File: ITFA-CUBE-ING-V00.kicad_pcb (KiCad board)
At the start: 2 copper layers, 90.2 x 95.9 mm, 34 parts, among them J1 Conn_01x04, U1 STM32H743VITx, U2 W25Q128JVS, Y1 25MHz 10pF, Y2 32.768K 7pF

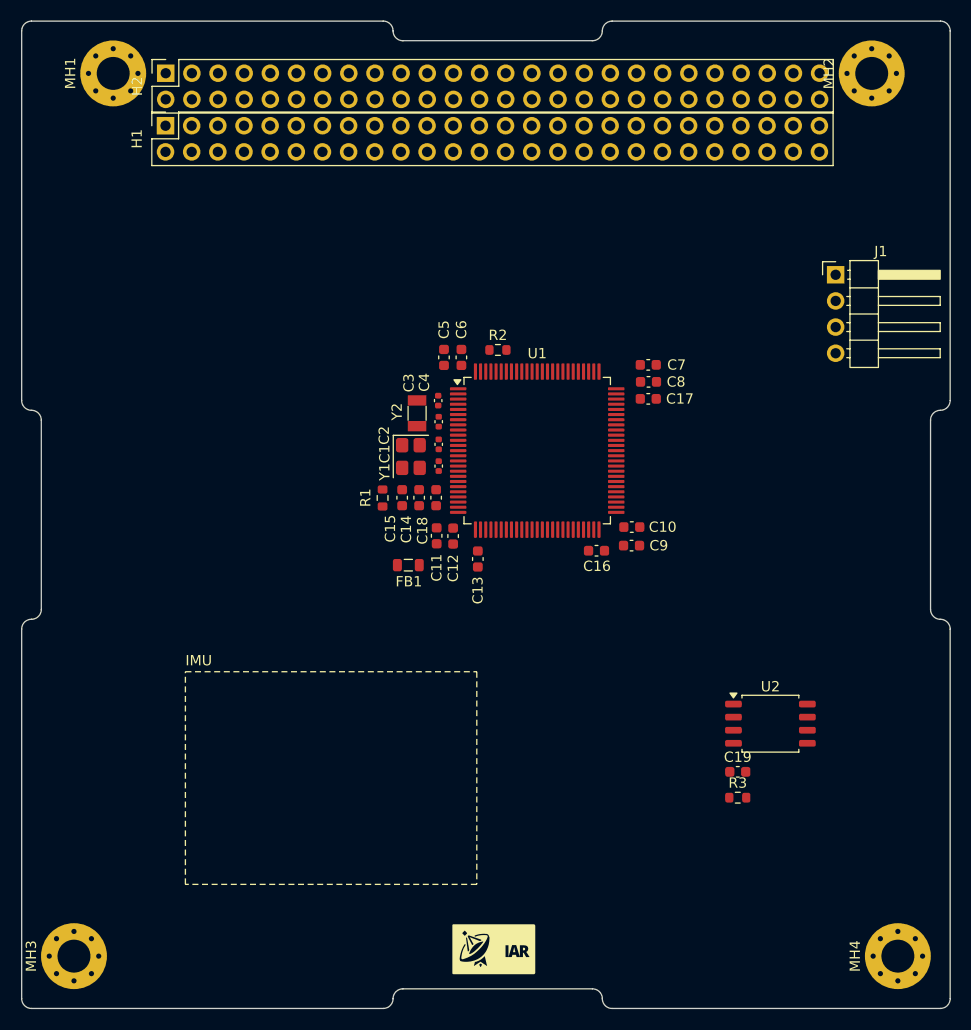
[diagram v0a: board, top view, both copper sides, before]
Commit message: Avance uc
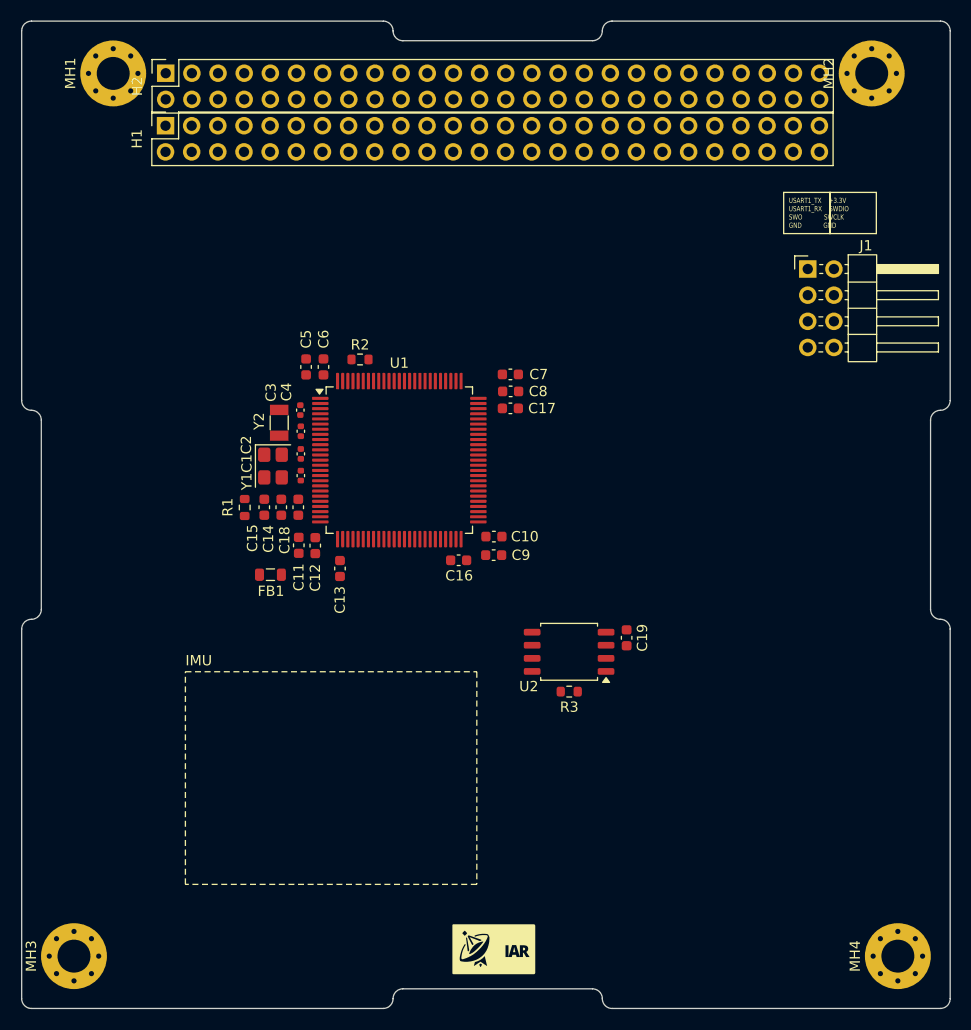
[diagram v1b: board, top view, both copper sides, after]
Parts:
- J1: value Conn_01x04 -> Conn_02x04_Odd_Even; footprint Connector_PinHeader_2.54mm:PinHeader_1x04_P2.54mm_Horizontal -> Connector_PinHeader_2.54mm:PinHeader_2x04_P2.54mm_Horizontal
- moved U2 20.8 mm to (139.8, 106.1), turned to 180 degrees
- moved R3 19.3 mm to (139.8, 110.0), turned to 180 degrees
- moved C19 16.9 mm to (145.4, 104.7), turned to 90 degrees
- moved C10 13.4 mm to (132.5, 94.9)
- moved C7 13.4 mm to (134.1, 79.2)
- moved C16 13.4 mm to (129.0, 97.2)
- moved C17 13.4 mm to (134.1, 82.5)
- moved C8 13.4 mm to (134.1, 80.8)
- moved C9 13.4 mm to (132.4, 96.7)
- moved R2 13.4 mm to (119.5, 77.7)
- moved U1 13.4 mm to (123.3, 87.5)
- moved C1 13.4 mm to (113.7, 86.9)
- moved C4 13.4 mm to (113.7, 82.6)
- moved C11 13.4 mm to (113.5, 95.8)
- moved C13 13.4 mm to (117.5, 98.0)
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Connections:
- net Net-(U1-PC14) renamed /RCC_OSC32_IN
- net Net-(U1-PC15) renamed /RCC_OSC32_OUT
- H1 pad 10: SPI_1_MOSI -> unconnected-(H1-Pin_10-Pad10)
- H1 pad 11: SPI_1_SCK -> unconnected-(H1-Pin_11-Pad11)
- H1 pad 12: SPI_1_MISO -> unconnected-(H1-Pin_12-Pad12)
- H1 pad 13: UART_1_TX -> unconnected-(H1-Pin_13-Pad13)
- H1 pad 14: UART_1_CTS -> unconnected-(H1-Pin_14-Pad14)
- H1 pad 15: UART_1_RX -> unconnected-(H1-Pin_15-Pad15)
- H1 pad 16: UART_1_RST -> unconnected-(H1-Pin_16-Pad16)
- H1 pad 17: UART_RCS_1_TX -> unconnected-(H1-Pin_17-Pad17)
- H1 pad 18: UART_RCS_1_CTS -> unconnected-(H1-Pin_18-Pad18)
- H1 pad 19: UART_RCS_1_RX -> unconnected-(H1-Pin_19-Pad19)
- H1 pad 20: UART_RCS_1_RST -> unconnected-(H1-Pin_20-Pad20)
- H1 pad 21: I2C_1_SCL -> unconnected-(H1-Pin_21-Pad21)
- H1 pad 22: I2C_1_SDA -> unconnected-(H1-Pin_22-Pad22)
- H1 pad 23: CAN_1_P -> unconnected-(H1-Pin_23-Pad23)
- H1 pad 24: CAN_1_N -> unconnected-(H1-Pin_24-Pad24)
- H1 pad 25: GLO_SYNC -> unconnected-(H1-Pin_25-Pad25)
- H1 pad 26: GLO_FAULT -> unconnected-(H1-Pin_26-Pad26)
- H1 pad 27: CPU_WD_1 -> unconnected-(H1-Pin_27-Pad27)
- H1 pad 30: CPU_MODE -> unconnected-(H1-Pin_30-Pad30)
- H1 pad 35: GLO_KS_1 -> unconnected-(H1-Pin_35-Pad35)
- H1 pad 39: USER_3_1 -> unconnected-(H1-Pin_39-Pad39)
- H1 pad 40: USER_3_2 -> unconnected-(H1-Pin_40-Pad40)
- H1 pad 41: USER_3_3 -> unconnected-(H1-Pin_41-Pad41)
- H1 pad 42: USER_3_4 -> unconnected-(H1-Pin_42-Pad42)
- H1 pad 43: USER_5_1 -> unconnected-(H1-Pin_43-Pad43)
- H1 pad 44: USER_5_2 -> unconnected-(H1-Pin_44-Pad44)
- H1 pad 45: USER_5_3 -> unconnected-(H1-Pin_45-Pad45)
- H1 pad 46: USER_5_4 -> unconnected-(H1-Pin_46-Pad46)
- H1 pad 5: USER_1_1 -> unconnected-(H1-Pin_5-Pad5)
- H1 pad 6: USER_1_2 -> unconnected-(H1-Pin_6-Pad6)
- H1 pad 7: SPI_1_CS2 -> unconnected-(H1-Pin_7-Pad7)
- H1 pad 8: USER_1_4 -> unconnected-(H1-Pin_8-Pad8)
- H1 pad 9: SPI_1_CS1 -> unconnected-(H1-Pin_9-Pad9)
- H2 pad 10: SPI_2_MOSI -> unconnected-(H2-Pin_10-Pad10)
- H2 pad 11: SPI_2_SCK -> unconnected-(H2-Pin_11-Pad11)
- H2 pad 12: SPI_2_MISO -> unconnected-(H2-Pin_12-Pad12)
- H2 pad 13: UART_2_TX -> unconnected-(H2-Pin_13-Pad13)
- H2 pad 14: UART_2_CTS -> unconnected-(H2-Pin_14-Pad14)
- H2 pad 15: UART_2_RX -> unconnected-(H2-Pin_15-Pad15)
- H2 pad 16: UART_2_RST -> unconnected-(H2-Pin_16-Pad16)
- H2 pad 17: UART_RCS_2_TX -> unconnected-(H2-Pin_17-Pad17)
- H2 pad 18: UART_RCS_2_CTS -> unconnected-(H2-Pin_18-Pad18)
- H2 pad 19: UART_RCS_2_RX -> unconnected-(H2-Pin_19-Pad19)
- H2 pad 20: UART_RCS_2_RST -> unconnected-(H2-Pin_20-Pad20)
- H2 pad 21: I2C_2_SCL -> unconnected-(H2-Pin_21-Pad21)
- H2 pad 22: I2C_2_SDA -> unconnected-(H2-Pin_22-Pad22)
- H2 pad 23: CAN_2_P -> unconnected-(H2-Pin_23-Pad23)
- H2 pad 24: CAN_2_N -> unconnected-(H2-Pin_24-Pad24)
- H2 pad 25: SUP_5V -> unconnected-(H2-Pin_25-Pad25)
- H2 pad 26: SUP_5V -> unconnected-(H2-Pin_26-Pad26)
- H2 pad 27: SUP_3V3 -> unconnected-(H2-Pin_27-Pad27)
- H2 pad 28: SUP_3V3 -> unconnected-(H2-Pin_28-Pad28)
- H2 pad 39: USER_4_1 -> unconnected-(H2-Pin_39-Pad39)
- H2 pad 40: USER_4_2 -> unconnected-(H2-Pin_40-Pad40)
- H2 pad 41: USER_4_3 -> unconnected-(H2-Pin_41-Pad41)
- H2 pad 42: USER_4_4 -> unconnected-(H2-Pin_42-Pad42)
- H2 pad 43: USER_6_1 -> unconnected-(H2-Pin_43-Pad43)
- H2 pad 44: USER_6_2 -> unconnected-(H2-Pin_44-Pad44)
- H2 pad 47: USER_6_3 -> unconnected-(H2-Pin_47-Pad47)
- H2 pad 48: USER_6_4 -> unconnected-(H2-Pin_48-Pad48)
- H2 pad 5: USER_2_1 -> unconnected-(H2-Pin_5-Pad5)
- H2 pad 6: USER_2_2 -> unconnected-(H2-Pin_6-Pad6)
- H2 pad 7: SPI_2_CS2 -> unconnected-(H2-Pin_7-Pad7)
- H2 pad 8: USER_2_4 -> unconnected-(H2-Pin_8-Pad8)
- H2 pad 9: SPI_2_CS1 -> unconnected-(H2-Pin_9-Pad9)
- J1 pad 1: +3.3V -> /USART1_TX
- J1 pad 2: /SWDIO -> +3.3V
- J1 pad 3: /SWCLK -> /USART1_RX
- J1 pad 4: GND -> /SWDIO
- R3 pad 1: /SPI_Flash_CS -> /SPI1_Flash1_CS
- U1 pad 1: unconnected-(U1-PE2-Pad1) -> /SPI4_CLK
- U1 pad 24: unconnected-(U1-PA2-Pad24) -> /USART2_TX
- U1 pad 25: unconnected-(U1-PA3-Pad25) -> /USART2_RX
- U1 pad 28: unconnected-(U1-PA4-Pad28) -> /SPI1_Flash1_CS
- U1 pad 29: unconnected-(U1-PA5-Pad29) -> /SPI1_CLK
- U1 pad 30: unconnected-(U1-PA6-Pad30) -> /SPI1_MISO
- U1 pad 31: unconnected-(U1-PA7-Pad31) -> /SPI1_MOSI
- U1 pad 4: unconnected-(U1-PE5-Pad4) -> /SPI4_MISO
- U1 pad 46: unconnected-(U1-PB10-Pad46) -> /I2C2_SCL
- U1 pad 47: unconnected-(U1-PB11-Pad47) -> /I2C2_SDA
- U1 pad 5: unconnected-(U1-PE6-Pad5) -> /SPI4_MOSI
- U1 pad 68: unconnected-(U1-PA9-Pad68) -> /USART1_TX
- U1 pad 69: unconnected-(U1-PA10-Pad69) -> /USART1_RX
- U1 pad 89: unconnected-(U1-PB3-Pad89) -> /SWO
- U1 pad 92: unconnected-(U1-PB6-Pad92) -> /I2C1_SCL
- U1 pad 93: unconnected-(U1-PB7-Pad93) -> /I2C1_SDA
- U1 pad 95: unconnected-(U1-PB8-Pad95) -> /CAN1-
- U1 pad 96: unconnected-(U1-PB9-Pad96) -> /CAN1+
- U2 pad 1: /SPI_Flash_CS -> /SPI1_Flash1_CS
- U2 pad 2: /SPI_Flash_MISO -> /SPI1_MISO
- U2 pad 5: /SPI_Flash_MOSI -> /SPI1_MOSI
- U2 pad 6: /SPI_Flash_CLK -> /SPI1_CLK
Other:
- board text added: "Instituro Argentino de Radioastronomia (IAR) Instituto Tecnico Florentino Ameghino (ITFA) STM32 Cubesat Test Board PC104 - uC: STM32H743VIT6 - Flash: W25Q128JVS 128Mbit / 16MiB Serial Flash Memory, SPI. - IMU:"
- board text added: "USART1_TX +3.3V USART1_RX SWDIO SWO SWCLK GND GND"
- board text added: "V00 S/N:"
- board text removed: "V00"

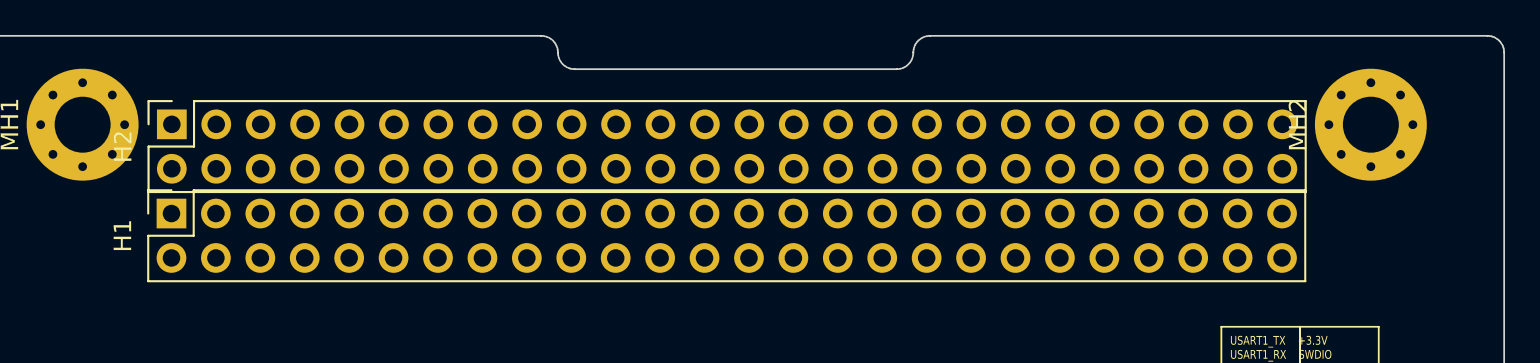
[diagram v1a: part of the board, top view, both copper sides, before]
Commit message: Actualizandon esquematico
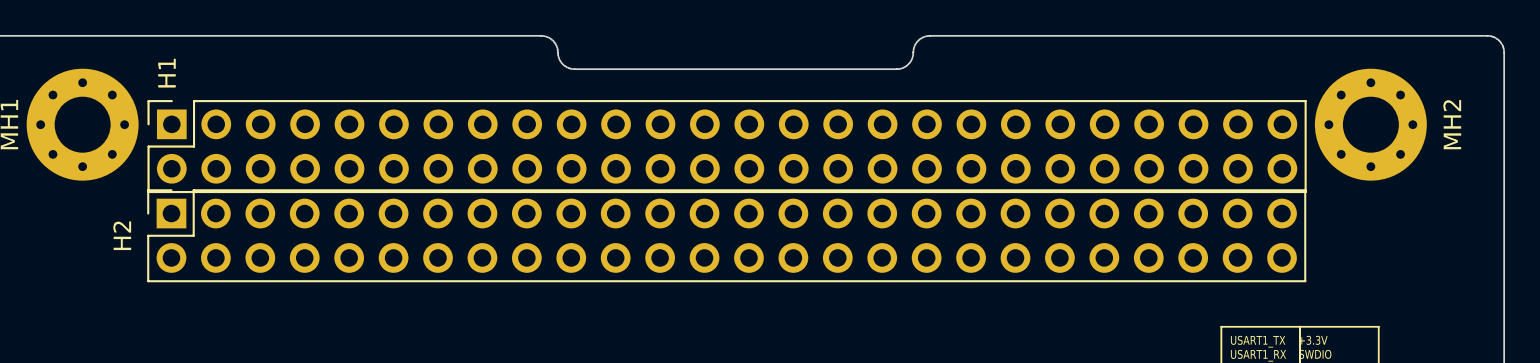
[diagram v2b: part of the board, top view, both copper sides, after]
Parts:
- moved H1 5.10 mm to (100.6, 49.9)
- moved H2 5.10 mm to (100.6, 55.0)
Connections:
- H1 pad 1: unconnected-(H1-Pin_1-Pad1) -> /DIG_A_01
- H1 pad 10: unconnected-(H1-Pin_10-Pad10) -> /DIG_A_10
- H1 pad 11: unconnected-(H1-Pin_11-Pad11) -> /SW2_VBAT
- H1 pad 12: unconnected-(H1-Pin_12-Pad12) -> /SW1_VBAT
- H1 pad 2: unconnected-(H1-Pin_2-Pad2) -> /DIG_A_02
- H1 pad 25: unconnected-(H1-Pin_25-Pad25) -> +5V
- H1 pad 26: unconnected-(H1-Pin_26-Pad26) -> +5V
- H1 pad 29: unconnected-(H1-Pin_29-Pad29) -> GND
- H1 pad 3: unconnected-(H1-Pin_3-Pad3) -> /DIG_A_03
- H1 pad 30: unconnected-(H1-Pin_30-Pad30) -> GND
- H1 pad 31: unconnected-(H1-Pin_31-Pad31) -> GND
- H1 pad 32: unconnected-(H1-Pin_32-Pad32) -> GND
- H1 pad 33: GND -> /ENA_PWR_5
- H1 pad 34: unconnected-(H1-Pin_34-Pad34) -> /PWR_5
- H1 pad 35: unconnected-(H1-Pin_35-Pad35) -> /ENA_PWR_6
- H1 pad 36: unconnected-(H1-Pin_36-Pad36) -> /PWR_6
- H1 pad 37: unconnected-(H1-Pin_37-Pad37) -> /ENA_PWR_7
- H1 pad 38: unconnected-(H1-Pin_38-Pad38) -> /PWR_7
- H1 pad 39: unconnected-(H1-Pin_39-Pad39) -> /ENA_PWR_8
- H1 pad 4: unconnected-(H1-Pin_4-Pad4) -> /DIG_A_04
- H1 pad 40: unconnected-(H1-Pin_40-Pad40) -> /PWR_8
- H1 pad 45: unconnected-(H1-Pin_45-Pad45) -> /VBAT
- H1 pad 46: unconnected-(H1-Pin_46-Pad46) -> /VBAT
- H1 pad 49: unconnected-(H1-Pin_49-Pad49) -> /RBF_OPEN
- H1 pad 5: unconnected-(H1-Pin_5-Pad5) -> /DIG_A_05
- H1 pad 50: unconnected-(H1-Pin_50-Pad50) -> /RBF_GND
- H1 pad 51: unconnected-(H1-Pin_51-Pad51) -> /KS_OPEN
- H1 pad 52: unconnected-(H1-Pin_52-Pad52) -> /KS_GND
- H1 pad 6: unconnected-(H1-Pin_6-Pad6) -> /DIG_A_06
- H1 pad 7: unconnected-(H1-Pin_7-Pad7) -> /DIG_A_07
- H1 pad 8: unconnected-(H1-Pin_8-Pad8) -> /DIG_A_08
- H1 pad 9: unconnected-(H1-Pin_9-Pad9) -> /DIG_A_09
- H2 pad 1: unconnected-(H2-Pin_1-Pad1) -> /CAN_A_L
- H2 pad 10: unconnected-(H2-Pin_10-Pad10) -> /SPI_A_MOSI
- H2 pad 11: unconnected-(H2-Pin_11-Pad11) -> /SPI_A_CLK
- H2 pad 12: unconnected-(H2-Pin_12-Pad12) -> /SPI_A_MISO
- H2 pad 13: unconnected-(H2-Pin_13-Pad13) -> /UART_A_TX
- H2 pad 15: unconnected-(H2-Pin_15-Pad15) -> /UART_A_RX
- H2 pad 2: unconnected-(H2-Pin_2-Pad2) -> /CAN_B_L
- H2 pad 21: unconnected-(H2-Pin_21-Pad21) -> /I2C_B_SCL
- H2 pad 22: unconnected-(H2-Pin_22-Pad22) -> /UART_B_TX
- H2 pad 23: unconnected-(H2-Pin_23-Pad23) -> /I2C_B_SDA
- H2 pad 24: unconnected-(H2-Pin_24-Pad24) -> /UART_B_RX
- H2 pad 25: unconnected-(H2-Pin_25-Pad25) -> +5V
- H2 pad 26: unconnected-(H2-Pin_26-Pad26) -> +5V
- H2 pad 29: GND -> unconnected-(H2-Pin_29-Pad29)
- H2 pad 3: unconnected-(H2-Pin_3-Pad3) -> /CAN_A_H
- H2 pad 30: GND -> unconnected-(H2-Pin_30-Pad30)
- H2 pad 32: GND -> unconnected-(H2-Pin_32-Pad32)
- H2 pad 33: unconnected-(H2-Pin_33-Pad33) -> GND
- H2 pad 34: unconnected-(H2-Pin_34-Pad34) -> GND
- H2 pad 35: unconnected-(H2-Pin_35-Pad35) -> GND
- H2 pad 36: unconnected-(H2-Pin_36-Pad36) -> GND
- H2 pad 4: unconnected-(H2-Pin_4-Pad4) -> /CAN_B_H
- H2 pad 41: unconnected-(H2-Pin_41-Pad41) -> /I2C_A_SDA
- H2 pad 43: unconnected-(H2-Pin_43-Pad43) -> /I2C_A_SCL
- H2 pad 45: unconnected-(H2-Pin_45-Pad45) -> /ENA_PWR_1
- H2 pad 46: unconnected-(H2-Pin_46-Pad46) -> +3.3V
- H2 pad 47: unconnected-(H2-Pin_47-Pad47) -> /ENA_PWR_2
- H2 pad 48: unconnected-(H2-Pin_48-Pad48) -> /PWR_2
- H2 pad 49: unconnected-(H2-Pin_49-Pad49) -> /ENA_PWR_3
- H2 pad 5: unconnected-(H2-Pin_5-Pad5) -> /UART_C_TX
- H2 pad 50: unconnected-(H2-Pin_50-Pad50) -> /PWR_3
- H2 pad 51: unconnected-(H2-Pin_51-Pad51) -> /ENA_PWR_4
- H2 pad 52: unconnected-(H2-Pin_52-Pad52) -> /PWR_4
- H2 pad 6: unconnected-(H2-Pin_6-Pad6) -> /UART_D_TX
- H2 pad 7: unconnected-(H2-Pin_7-Pad7) -> /UART_C_RX
- H2 pad 8: unconnected-(H2-Pin_8-Pad8) -> /UART_D_RX
- H2 pad 9: unconnected-(H2-Pin_9-Pad9) -> /SPI_A_CS
- U1 pad 2: unconnected-(U1-PE3-Pad2) -> /SPI4_CS
- U1 pad 32: unconnected-(U1-PC4-Pad32) -> /PC4
- U1 pad 33: unconnected-(U1-PC5-Pad33) -> /PC5
- U1 pad 63: unconnected-(U1-PC6-Pad63) -> /PC6
- U1 pad 64: unconnected-(U1-PC7-Pad64) -> /PC7
- U1 pad 65: unconnected-(U1-PC8-Pad65) -> /PC8
- U1 pad 66: unconnected-(U1-PC9-Pad66) -> /PC9
- U1 pad 7: unconnected-(U1-PC13-Pad7) -> /PC13
- U1 pad 78: unconnected-(U1-PC10-Pad78) -> /PC10
- U1 pad 79: unconnected-(U1-PC11-Pad79) -> /PC11
- U1 pad 80: unconnected-(U1-PC12-Pad80) -> /PC12
